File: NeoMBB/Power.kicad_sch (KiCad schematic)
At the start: 37 parts

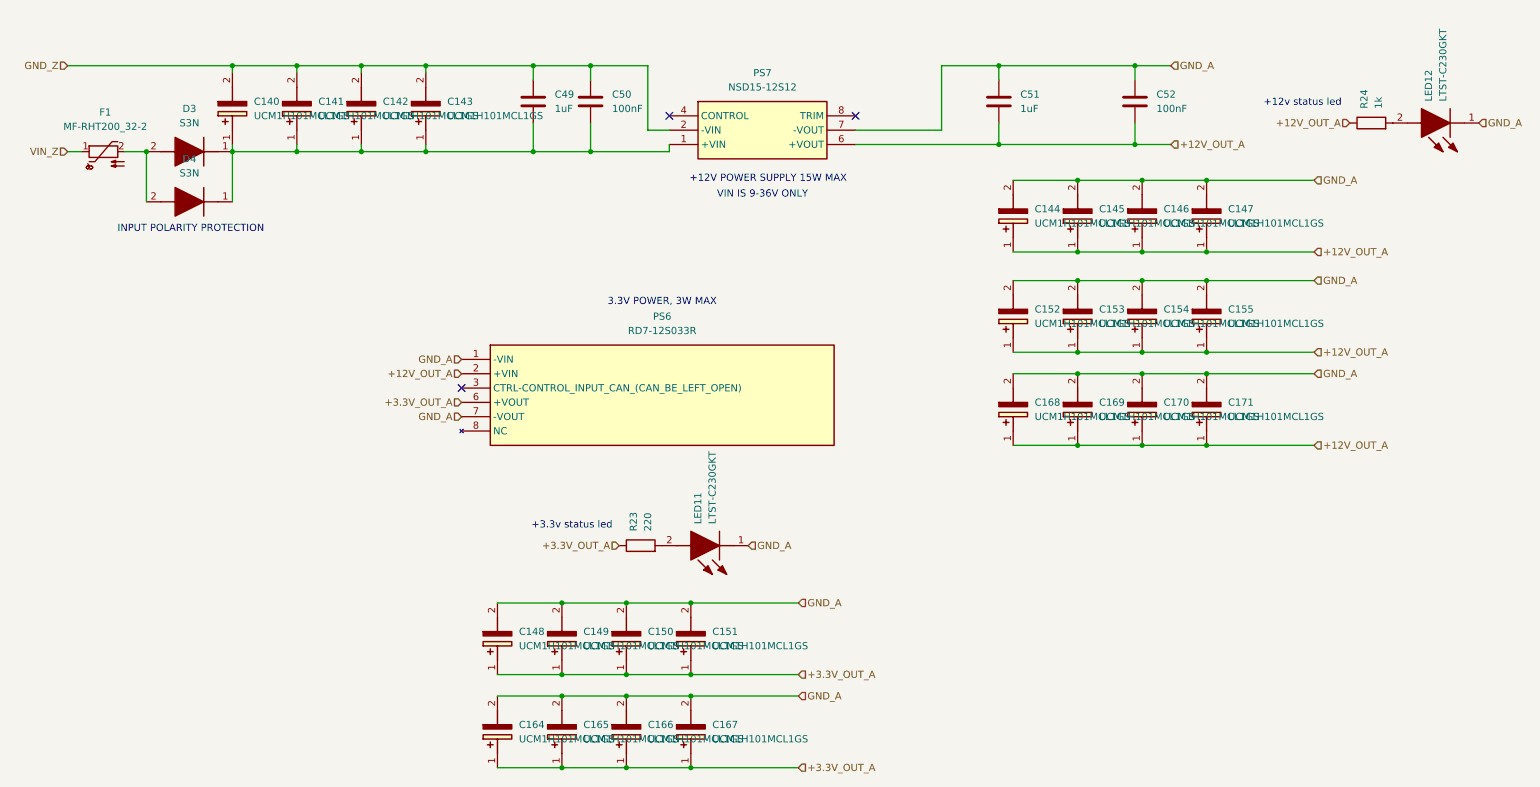
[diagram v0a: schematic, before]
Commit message: MBB Reverse engineering bs
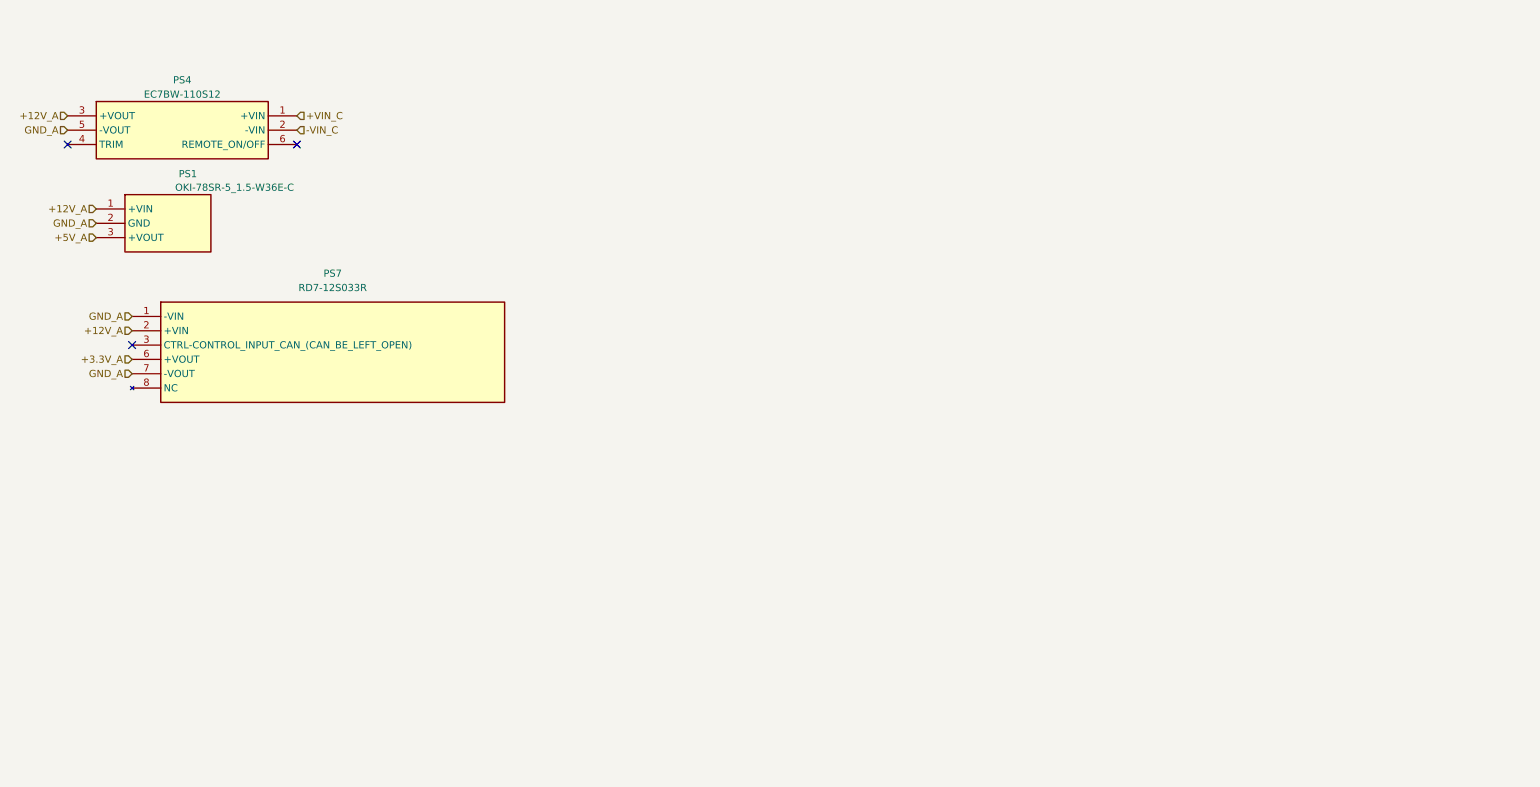
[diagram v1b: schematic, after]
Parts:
- removed C140, C141, C142, C143, C144, C145, C146, C147, C148, C149, C150, C151, C152, C153, C154, C155, C164, C165, C166, C167, C168, C169, C170, C171: UCM1H101MCL1GS, InverterCom:CAPAE660X800N, symbol InverterCom:UCM1H101MCL1GS
- removed C49, C51: 1uF, Capacitor_SMD:C_1210_3225Metric_Pad1.33x2.70mm_HandSolder, symbol Device:C
- removed C50, C52: 100nF, Capacitor_SMD:C_1210_3225Metric_Pad1.33x2.70mm_HandSolder, symbol Device:C
- removed D3, D4: S3N, InverterCom:DIOM8059X265N, symbol InverterCom:S3N
- removed F1: MF-RHT200_32-2, InverterCom:MFRHT200322, symbol InverterCom:MF-RHT200_32-2
- removed LED11, LED12: LTST-C230GKT, InverterCom:LEDC3216X120N, symbol InverterCom:LTST-C230GKT
- removed PS6: RD7-12S033R, InverterCom:RD712S033R, symbol InverterCom:RD7-12S033R
- removed PS7: NSD15-12S12, InverterCom:NSD1512S12, symbol InverterCom:NSD15-12S12
- removed R23: 220, Resistor_SMD:R_1210_3225Metric_Pad1.30x2.65mm_HandSolder, symbol Device:R
- removed R24: 1k, Resistor_SMD:R_1210_3225Metric_Pad1.30x2.65mm_HandSolder, symbol Device:R
- added PS1: OKI-78SR-5_1.5-W36E-C, InverterCom:OKI78SR515W36EC, symbol InverterCom:OKI-78SR-5_1.5-W36E-C
- added PS4: EC7BW-110S12, EC7BW110S12, symbol InverterCom:EC7BW-110S12
- added PS7: RD7-12S033R, RD712S033R, symbol InverterCom:RD7-12S033R
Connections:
- net GND_A: now also PS1.2 (GND), PS4.5 (-VOUT), PS7.1 (-VIN), PS7.7 (-VOUT)
- new net +12V_A: PS1.1 (+VIN), PS4.3 (+VOUT), PS7.2 (+VIN)
- new net +3.3V_A: PS7.6 (+VOUT)
- new net +5V_A: PS1.3 (+VOUT)
- new net +VIN_C: PS4.1 (+VIN)
- new net -VIN_C: PS4.2 (-VIN)
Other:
- note removed: "+12V POWER SUPPLY 15W MAX"
- note removed: "+12v status led"
- note removed: "+3.3v status led"
- note removed: "3.3V POWER, 3W MAX"
- note removed: "INPUT POLARITY PROTECTION"
- note removed: "VIN IS 9-36V ONLY"
